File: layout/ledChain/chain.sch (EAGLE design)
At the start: 29 parts, among them IC2 FT232RL, P1 FSM4JSMA-SMD, T1 BC848, T2 BC848

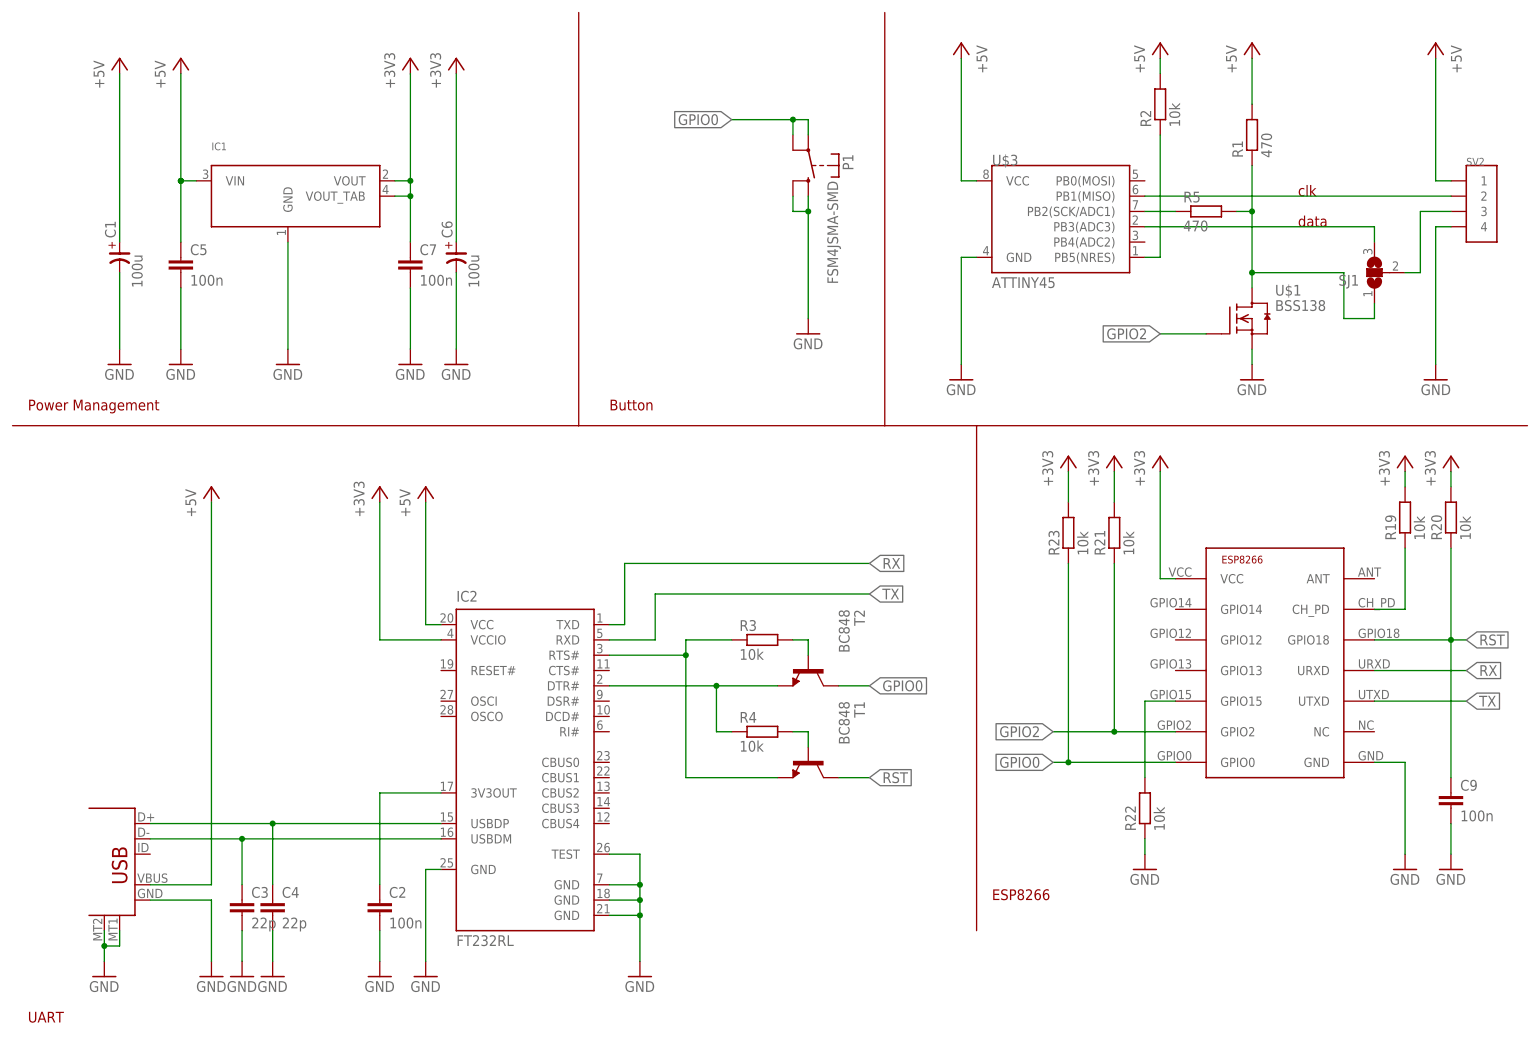
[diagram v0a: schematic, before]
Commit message: not quite their
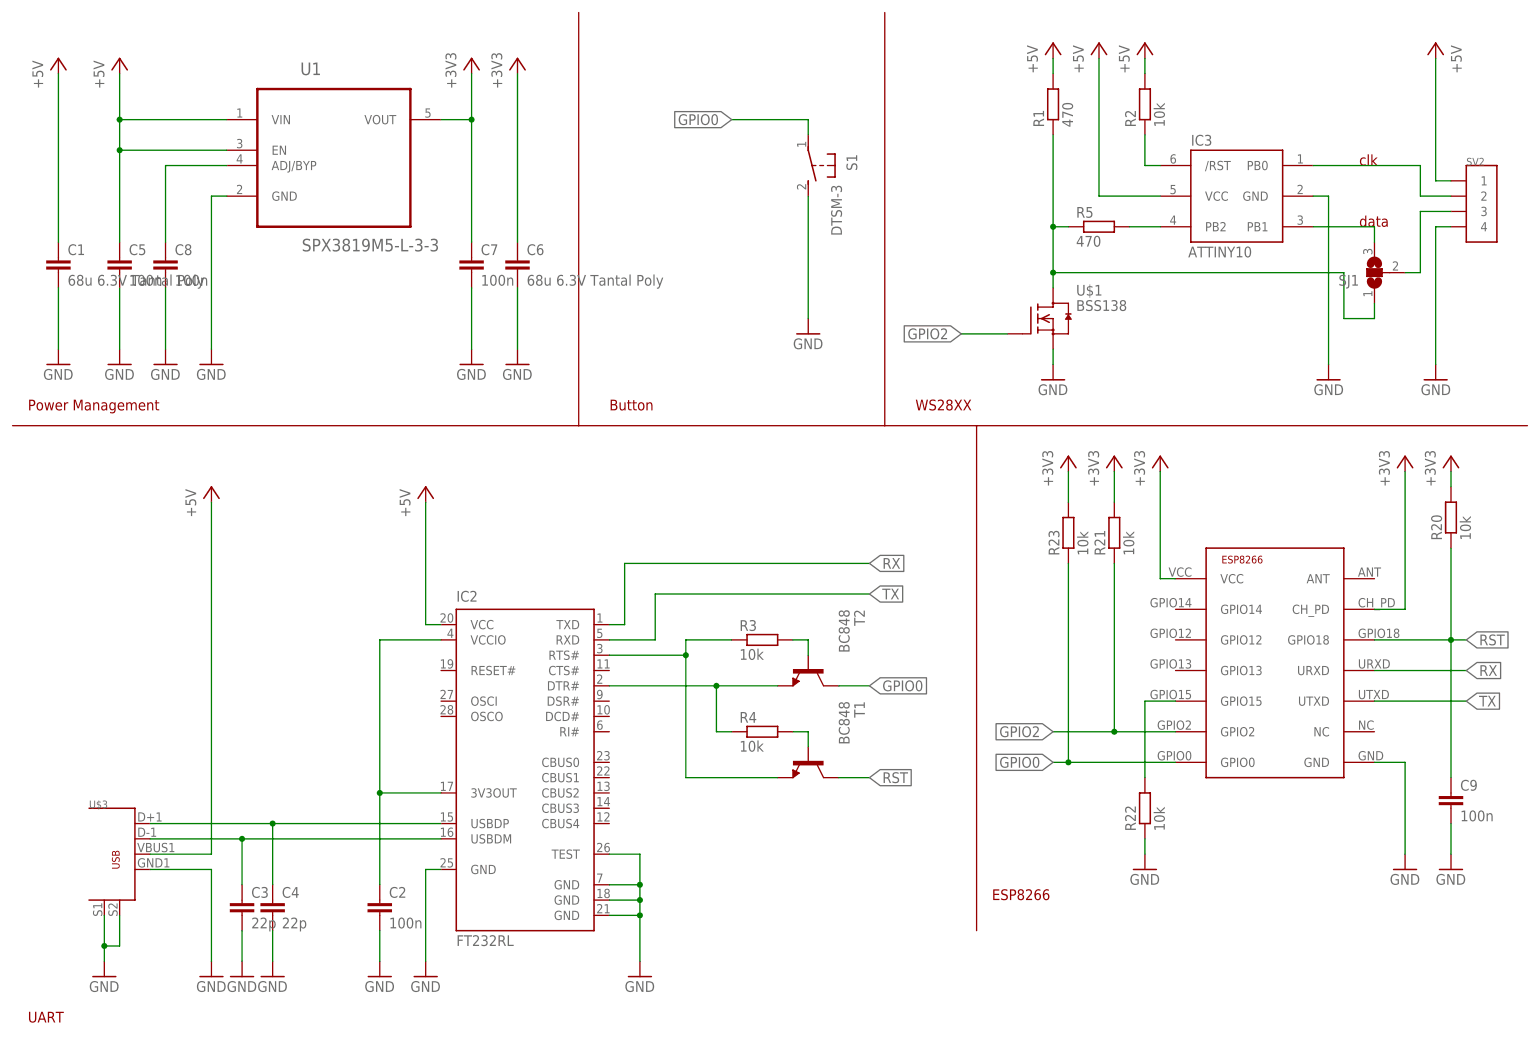
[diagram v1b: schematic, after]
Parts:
- removed IC1: (no value), sid:LM1117IMP
- removed P1: FSM4JSMA-SMD, switch-misc:FSM4JSMA-SMD
- removed R19: 10k, rcl-2:R-EU_R0603
- removed U$40: USB-B, sid:USB-B
- added C8: 100n, rcl:C-EUC0603
- added IC3: ATTINY10, adafruit:ATTINY10
- added S1: DTSM-3, switch-tact:DTSM-3
- added U1: SPX3819M5-L-3-3, ESP8266-2:SPX3819M5-L-3-3
- C1, C6: value 100u -> 68u 6.3V Tantal Poly; device cap-master:CP-7343-TE-D -> rcl-2:C-EUC0805
- U$3: value ATTINY45 -> USB-MALE-SMT; device SparkFun:ATTINY45 -> sid:USB-MALE-SMT
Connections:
- removed net N$12: C2.1, IC2.3V3OUT
- removed net N$2: R19.1, U$2.CH_PD
- new net N$15: C2.1, IC2.3V3OUT, IC2.VCCIO
- new net N$17: C8.1, U1.ADJ/BYP
- net +3V3: now also C6.1, U$2.CH_PD, U1.VOUT; no longer C6.+, IC1.VOUT, IC1.VOUT_TAB, IC2.VCCIO, R19.2
- net +5V: now also C1.1, IC3.VCC, U$3.VBUS, U1.EN, U1.VIN; no longer C1.+, IC1.VIN, U$3.VCC, U$40.VBUS
- net GND: now also C1.2, C6.2, C8.2, IC3.GND, S1.2, U$3.S1, U$3.S2, U1.GND; no longer C1.-, C6.-, IC1.GND, P1.S, P1.S@1, U$40.GND, U$40.P$1, U$40.P$2
- net GPIO0: now also S1.1; no longer P1.P, P1.P@1
- net N$10: now also IC3.PB0, SV2.2; no longer R5.1, U$3.PB2(SCK/ADC1)
- net N$11: now also IC3./RST, R2.1; no longer SV2.2, U$3.PB1(MISO)
- net N$13: now also IC3.PB1; no longer U$3.PB3(ADC3)
- net N$14: now also R5.1; no longer R5.2
- net N$3: now also U$3.D+; no longer U$40.D+
- net N$4: now also U$3.D-; no longer U$40.D-
- net N$6: now also IC3.PB2, R5.2; no longer R2.1, U$3.PB5(NRES)
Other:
- note added: "WS28XX"
- moved on the sheet: C5, C7, R1, R2, R5, U$1
